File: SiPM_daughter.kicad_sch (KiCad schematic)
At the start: 3 parts, among them J1 Conn_01x02, J4 Conn_01x02

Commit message: update pin connector size
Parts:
- J1, J4: footprint Connector_PinHeader_1.27mm:PinHeader_1x02_P1.27mm_Vertical -> Connector_PinHeader_2.54mm:PinHeader_1x02_P2.54mm_Vertical
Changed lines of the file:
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@@
       (effects (font (size 1.27 1.27)))
     )
-    (property "Footprint" "Connector_PinHeader_1.27mm:PinHeader_1x02_P1.27mm_Vertical" (at 147.574 113.03 0)
+    (property "Footprint" "Connector_PinHeader_2.54mm:PinHeader_1x02_P2.54mm_Vertical" (at 147.574 113.03 0)
       (effects (font (size 1.27 1.27)) hide)
     )
@@
       (effects (font (size 1.27 1.27)))
     )
-    (property "Footprint" "Connector_PinHeader_1.27mm:PinHeader_1x02_P1.27mm_Vertical" (at 124.206 113.03 0)
+    (property "Footprint" "Connector_PinHeader_2.54mm:PinHeader_1x02_P2.54mm_Vertical" (at 124.206 113.03 0)
       (effects (font (size 1.27 1.27)) hide)
     )

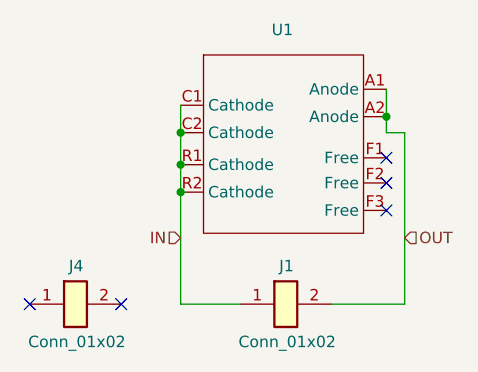
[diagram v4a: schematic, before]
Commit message: 2 SiPM AND Trigger Board
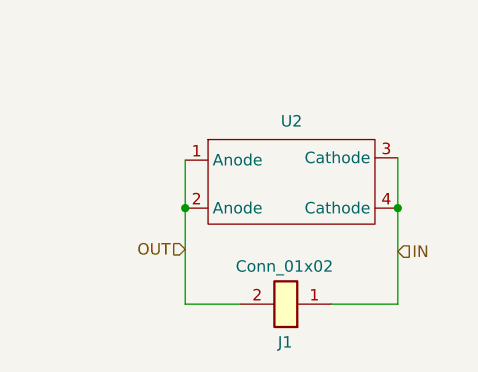
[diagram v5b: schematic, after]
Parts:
- removed J4: Conn_01x02, Connector_PinHeader_2.54mm:PinHeader_1x02_P2.54mm_Vertical, symbol EOS_library:Conn_01x02
- removed U1: ~, EOS_library:AFBR-S4N33C013, symbol EOS_library:AFBR-S4N33C013
- added U2: ~, EOS_library:AFBR-S4K11C0125B, symbol Eos_Library:AFBR-S4K11C0125B
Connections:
- net IN: now also U2.3 (Cathode), U2.4 (Cathode)
- net OUT: now also U2.1 (Anode), U2.2 (Anode)
- no-connect marks 5 -> 0
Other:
- moved on the sheet: J1
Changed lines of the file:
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@@
 (kicad_sch (version 20230121) (generator eeschema)
   (paper "A4")
-  (junction (at 158.75 93.472) (diameter 0) (color 0 0 0 0)
+  (junction (at 136.398 103.632) (diameter 0) (color 0 0 0 0)
   )
-  (junction (at 135.89 95.25) (diameter 0) (color 0 0 0 0)
+  (junction (at 160.02 103.632) (diameter 0) (color 0 0 0 0)
   )
-  (junction (at 135.89 98.806) (diameter 0) (color 0 0 0 0)
-  )
-  (junction (at 135.89 101.854) (diameter 0) (color 0 0 0 0)
-  )
-  (no_connect (at 158.75 103.886))
-  (no_connect (at 158.75 100.838))
-  (no_connect (at 119.126 114.3))
-  (no_connect (at 158.75 98.044))
-  (no_connect (at 129.286 114.3))
-  (wire (pts (xy 135.89 92.202) (xy 135.89 95.25))
+  (wire (pts (xy 160.02 114.3) (xy 152.654 114.3))
     (stroke (width 0) (type default))
   )
-  (wire (pts (xy 158.75 95.25) (xy 160.782 95.25))
+  (wire (pts (xy 136.398 103.632) (xy 136.398 114.3))
     (stroke (width 0) (type default))
   )
-  (wire (pts (xy 158.75 93.472) (xy 158.75 95.25))
+  (wire (pts (xy 136.398 114.3) (xy 142.494 114.3))
     (stroke (width 0) (type default))
   )
-  (wire (pts (xy 158.75 90.424) (xy 158.75 93.472))
+  (wire (pts (xy 136.398 98.298) (xy 136.398 103.632))
     (stroke (width 0) (type default))
   )
-  (wire (pts (xy 135.89 95.25) (xy 135.89 98.806))
+  (wire (pts (xy 160.02 98.044) (xy 160.02 103.632))
     (stroke (width 0) (type default))
   )
-  (wire (pts (xy 135.89 101.854) (xy 135.89 114.3))
+  (wire (pts (xy 160.02 103.632) (xy 160.02 114.3))
     (stroke (width 0) (type default))
   )
-  (wire (pts (xy 160.782 114.3) (xy 152.654 114.3))
-    (stroke (width 0) (type default))
+  (hierarchical_label "OUT" (shape input) (at 136.398 108.204 180) (fields_autoplaced)
+    (effects (font (size 1.27 1.27)) (justify right))
   )
-  (wire (pts (xy 135.89 114.3) (xy 142.494 114.3))
-    (stroke (width 0) (type default))
-  )
-  (wire (pts (xy 135.89 98.806) (xy 135.89 101.854))
-    (stroke (width 0) (type default))
-  )
-  (wire (pts (xy 160.782 95.25) (xy 160.782 114.3))
-    (stroke (width 0) (type default))
-  )
-  (hierarchical_label "OUT" (shape input) (at 160.782 106.934 0) (fields_autoplaced)
+  (hierarchical_label "IN" (shape input) (at 160.02 108.458 0) (fields_autoplaced)
     (effects (font (size 1.27 1.27)) (justify left))
   )
-  (hierarchical_label "IN" (shape input) (at 135.89 106.934 180) (fields_autoplaced)
-    (effects (font (size 1.27 1.27)) (justify right))
-  )
-  (symbol (lib_id "EOS_library:Conn_01x02") (at 147.574 113.03 0) (unit 1)
+  (symbol (lib_id "EOS_library:Conn_01x02") (at 147.574 115.57 180) (unit 1)
     (in_bom yes) (on_board yes) (dnp no)
-    (property "Reference" "J1" (at 147.6502 110.0582 0)
+    (property "Reference" "J1" (at 147.4978 118.5418 0)
       (effects (font (size 1.27 1.27)))
     )
-    (property "Value" "Conn_01x02" (at 147.7264 118.491 0)
+    (property "Value" "Conn_01x02" (at 147.4216 110.109 0)
       (effects (font (size 1.27 1.27)))
     )
-    (property "Footprint" "Connector_PinHeader_2.54mm:PinHeader_1x02_P2.54mm_Vertical" (at 147.574 113.03 0)
+    (property "Footprint" "Connector_PinHeader_2.54mm:PinHeader_1x02_P2.54mm_Vertical" (at 147.574 115.57 0)
       (effects (font (size 1.27 1.27)) hide)
     )
-    (property "Datasheet" "~" (at 147.574 113.03 0)
+    (property "Datasheet" "~" (at 147.574 115.57 0)
       (effects (font (size 1.27 1.27)) hide)
     )
@@
           (reference "J1") (unit 1)
         )
+        (path "/35db8c63-fd46-4d81-b248-207e32fc4dfb/7365ae05-6dfb-4f58-9a2d-77b53471d536"
+          (reference "J6") (unit 1)
+        )
       )
     )
   )
-  (symbol (lib_id "EOS_library:AFBR-S4N33C013") (at 147.32 96.52 0) (unit 1)
-    (in_bom yes) (on_board yes) (dnp no)
-    (property "Reference" "U1" (at 147.193 83.82 0)
+  (symbol (lib_id "Eos_Library:AFBR-S4K11C0125B") (at 148.336 101.346 0) (unit 1)
+    (in_bom yes) (on_board yes) (dnp no) (fields_autoplaced)
+    (property "Reference" "U2" (at 148.209 93.98 0)
       (effects (font (size 1.27 1.27)))
     )
-    (property "Value" "~" (at 147.32 109.22 0)
+    (property "Value" "~" (at 148.336 101.346 0)
       (effects (font (size 1.27 1.27)))
     )
-    (property "Footprint" "EOS_library:AFBR-S4N33C013" (at 147.32 96.52 0)
+    (property "Footprint" "EOS_library:AFBR-S4K11C0125B" (at 148.336 101.346 0)
       (effects (font (size 1.27 1.27)) hide)
     )
-    (property "Datasheet" "" (at 147.32 96.52 0)
+    (property "Datasheet" "" (at 148.336 101.346 0)
       (effects (font (size 1.27 1.27)) hide)
     )
-    (pin "A1")
-    (pin "A2")
-    (pin "C1")
-    (pin "C2")
-    (pin "F1")
-    (pin "F2")
-    (pin "F3")
-    (pin "R1")
-    (pin "R2")
+    (pin "1")
+    (pin "2")
+    (pin "3")
+    (pin "4")
     (instances
       (project "SiPM_daughter"
         (path "/003e91a7-1682-47be-8bcb-0d42bc83000d"
-          (reference "U1") (unit 1)
+          (reference "U2") (unit 1)
         )
       )
       (project "eos_trigger_proto"
         (path "/35db8c63-fd46-4d81-b248-207e32fc4dfb/23e0edf2-5306-4a3c-8e49-3ebf9dd0f3c4"
-          (reference "U1") (unit 1)
+          (reference "U12") (unit 1)
+        )
+        (path "/35db8c63-fd46-4d81-b248-207e32fc4dfb/7365ae05-6dfb-4f58-9a2d-77b53471d536"
+          (reference "U13") (unit 1)
         )
       )
     )
   )
-  (symbol (lib_id "EOS_library:Conn_01x02") (at 124.206 113.03 0) (unit 1)
-    (in_bom yes) (on_board yes) (dnp no)
-    (property "Reference" "J4" (at 124.2822 110.0582 0)
-      (effects (font (size 1.27 1.27)))
-    )
-    (property "Value" "Conn_01x02" (at 124.3584 118.491 0)
-      (effects (font (size 1.27 1.27)))
-    )
-    (property "Footprint" "Connector_PinHeader_2.54mm:PinHeader_1x02_P2.54mm_Vertical" (at 124.206 113.03 0)
-      (effects (font (size 1.27 1.27)) hide)
-    )
-    (property "Datasheet" "~" (at 124.206 113.03 0)
-      (effects (font (size 1.27 1.27)) hide)
-    )
-    (pin "1")
-    (pin "2")
-    (instances
-      (project "SiPM_daughter"
-        (path "/003e91a7-1682-47be-8bcb-0d42bc83000d"
-          (reference "J4") (unit 1)
-        )
-      )
-      (project "eos_trigger_proto"
-        (path "/35db8c63-fd46-4d81-b248-207e32fc4dfb/23e0edf2-5306-4a3c-8e49-3ebf9dd0f3c4"
-          (reference "J4") (unit 1)
-        )
-      )
-    )
-  )
-  (sheet_instances
-    (path "/" (page "1"))
-  )
 )
